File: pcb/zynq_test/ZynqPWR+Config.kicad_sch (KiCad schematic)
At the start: 43 parts, among them SW601 PS_RST, SW602 PROG, U202 XC7Z020-2CLG400I

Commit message: finished diff of HDMI
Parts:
- C601, C604, C605: footprint (none) -> Capacitor_SMD:C_1210_3225Metric
- C632: footprint Capacitor_SMD:C_0402_1005Metric -> Capacitor_SMD:C_1210_3225Metric
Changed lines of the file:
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@@
 			)
 		)
-		(property "Footprint" ""
+		(property "Footprint" "Capacitor_SMD:C_1210_3225Metric"
 			(at 35.2552 83.82 0)
 			(effects
@@
 			)
 		)
-		(property "Footprint" "Capacitor_SMD:C_0402_1005Metric"
+		(property "Footprint" "Capacitor_SMD:C_1210_3225Metric"
 			(at 166.6748 39.37 0)
 			(effects
@@
 			)
 		)
-		(property "Footprint" ""
+		(property "Footprint" "Capacitor_SMD:C_1210_3225Metric"
 			(at 35.2552 62.23 0)
 			(effects
@@
 			)
 		)
-		(property "Footprint" ""
+		(property "Footprint" "Capacitor_SMD:C_1210_3225Metric"
 			(at 17.4752 105.41 0)
 			(effects

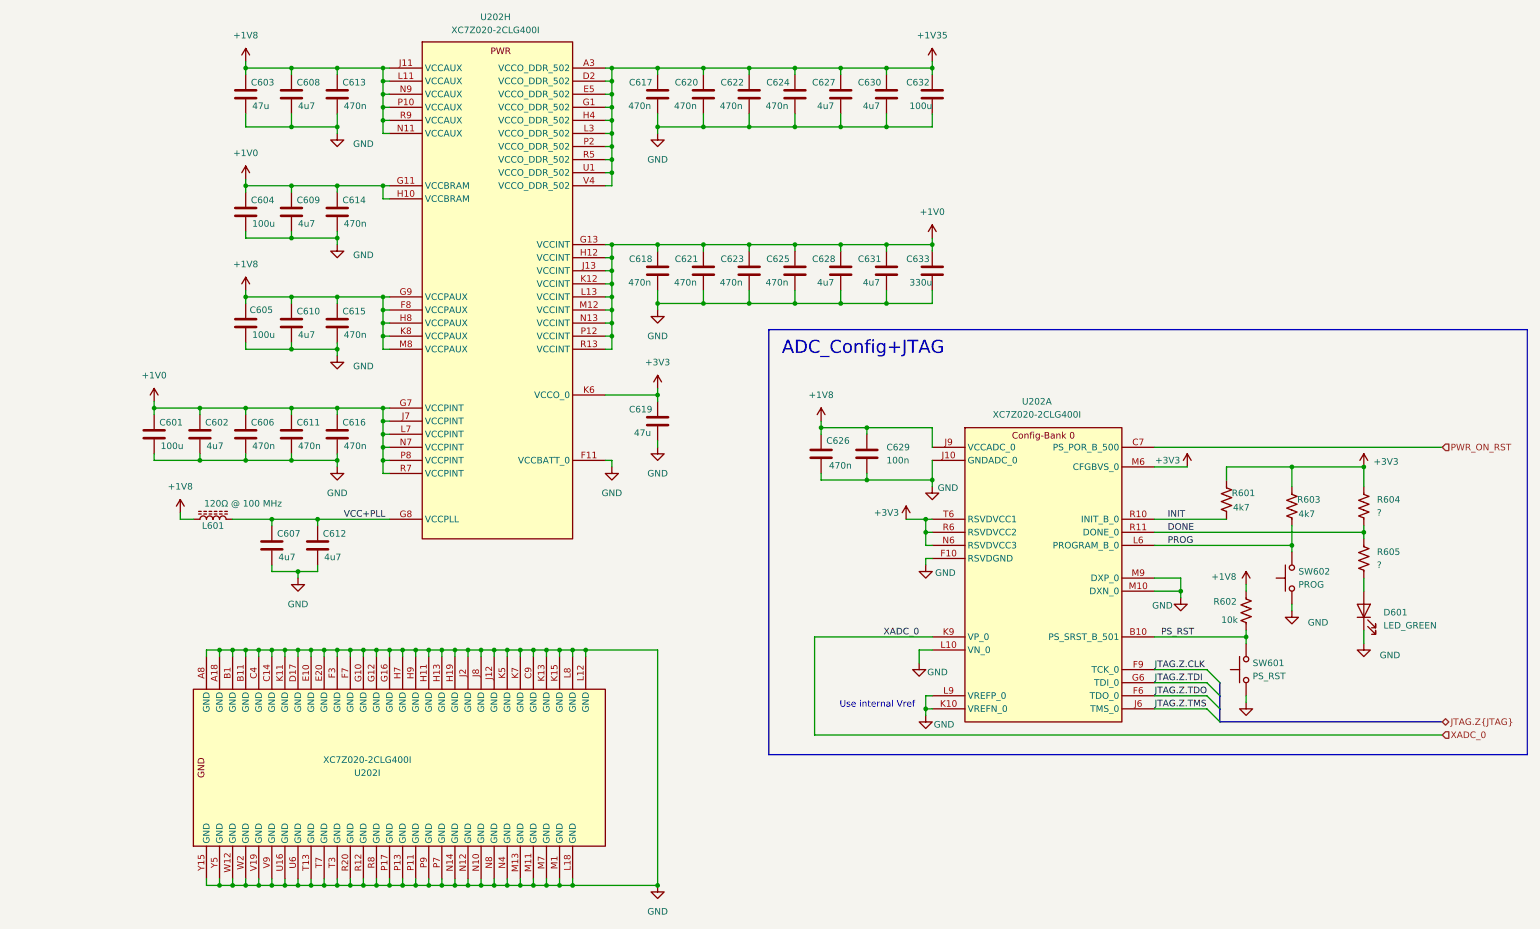
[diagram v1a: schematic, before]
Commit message: Almost done with BOM
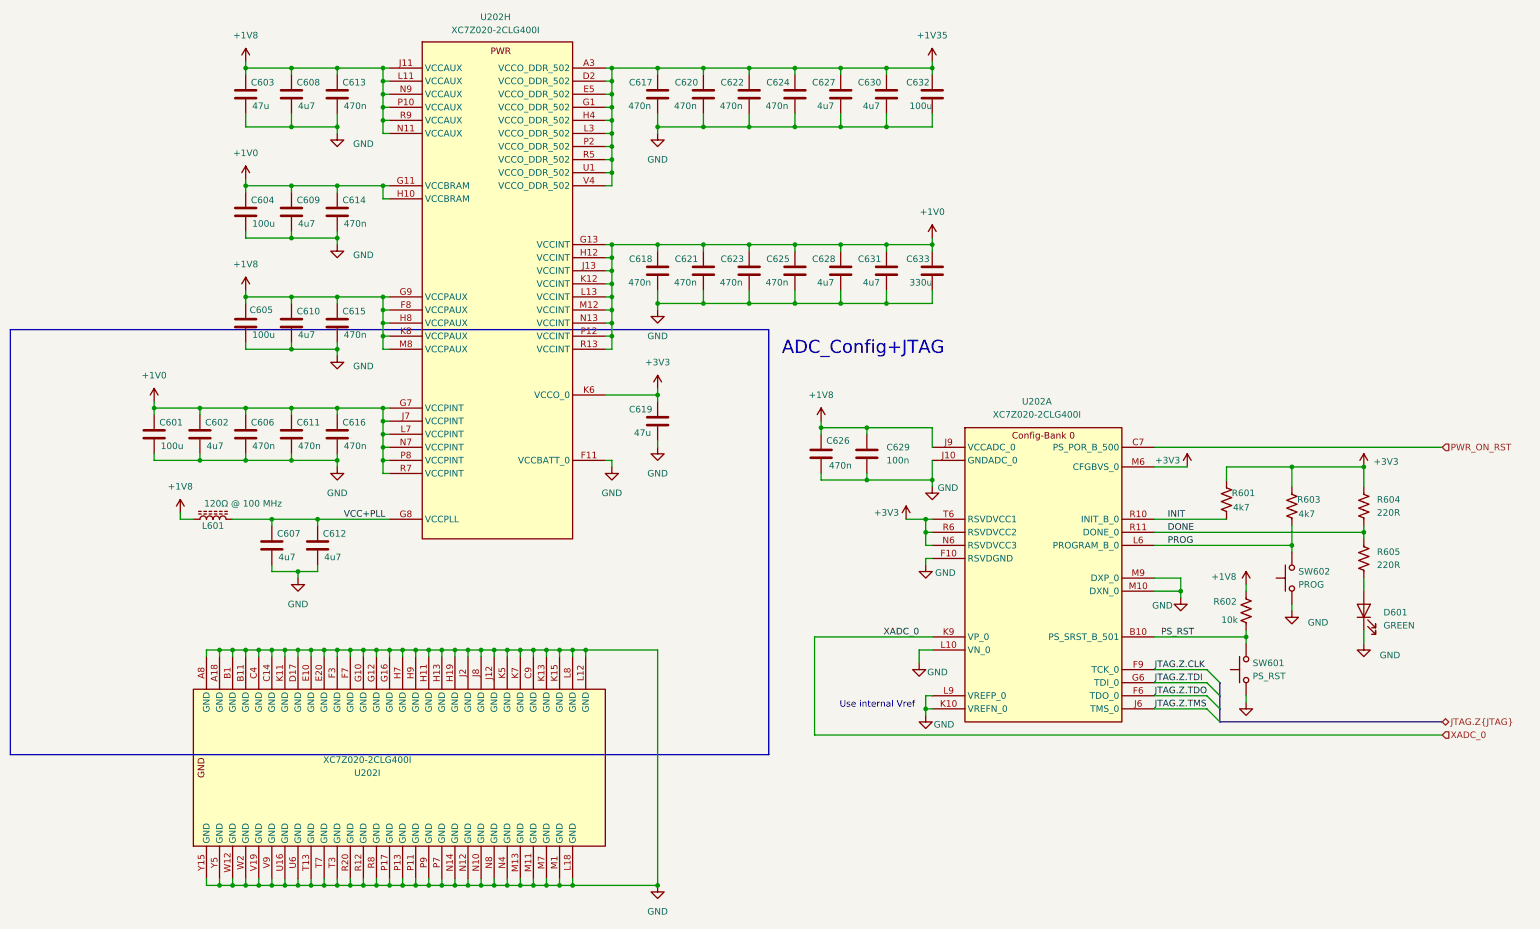
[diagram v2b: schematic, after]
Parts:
- C602, C606, C607, C608, C609, C610, C611, C612, C613, C614, C615, C616, C618, C621, C623, C625, C626, C628, C629, C631: footprint (none) -> Capacitor_SMD:C_0402_1005Metric
- C603, C619, C633: footprint (none) -> Capacitor_SMD:C_1210_3225Metric
- D601: value LED_GREEN -> GREEN; footprint (none) -> LED_SMD:LED_0805_2012Metric
- L601: footprint (none) -> Capacitor_SMD:C_0603_1608Metric
- R601, R602, R603: footprint (none) -> Resistor_SMD:R_0402_1005Metric
- R604, R605: value ? -> 220R; footprint (none) -> Resistor_SMD:R_0402_1005Metric
- SW601, SW602: footprint (none) -> Button_Switch_THT:SW_PUSH_1P1T_6x3.5mm_H4.3_APEM_MJTP1243
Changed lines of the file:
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@@
 	(rectangle
 		(start 135.89 81.28)
-		(end 283.21 163.83)
+		(end -11.43 163.83)
 		(stroke
 			(width 0)
@@
 			)
 		)
-		(property "Value" "?"
+		(property "Value" "220R"
 			(at 254 126.9999 0)
 			(effects
@@
 			)
 		)
-		(property "Footprint" ""
+		(property "Footprint" "Resistor_SMD:R_0402_1005Metric"
 			(at 252.476 125.984 90)
 			(effects
@@
 			)
 		)
-		(property "Footprint" ""
+		(property "Footprint" "Capacitor_SMD:C_0402_1005Metric"
 			(at 155.9052 109.22 0)
 			(effects
@@
 			)
 		)
-		(property "Footprint" ""
+		(property "Footprint" "Button_Switch_THT:SW_PUSH_1P1T_6x3.5mm_H4.3_APEM_MJTP1243"
 			(at 223.52 147.32 0)
 			(effects
@@
 			)
 		)
-		(property "Footprint" ""
+		(property "Footprint" "Capacitor_SMD:C_0402_1005Metric"
 			(at 147.0152 109.22 0)
 			(effects
@@
 			)
 		)
-		(property "Footprint" ""
+		(property "Footprint" "Capacitor_SMD:C_0402_1005Metric"
 			(at 53.0352 105.41 0)
 			(effects
@@
 			)
 		)
-		(property "Footprint" ""
+		(property "Footprint" "Button_Switch_THT:SW_PUSH_1P1T_6x3.5mm_H4.3_APEM_MJTP1243"
 			(at 232.41 129.54 0)
 			(effects
@@
 			)
 		)
-		(property "Footprint" ""
+		(property "Footprint" "Capacitor_SMD:C_0402_1005Metric"
 			(at 140.0048 73.66 0)
 			(effects
@@
 			)
 		)
-		(property "Footprint" ""
+		(property "Footprint" "Capacitor_SMD:C_1210_3225Metric"
 			(at 35.2552 39.37 0)
 			(effects
@@
 			)
 		)
-		(property "Footprint" ""
+		(property "Footprint" "Resistor_SMD:R_0402_1005Metric"
 			(at 225.806 114.554 90)
 			(effects
@@
 			)
 		)
-		(property "Footprint" ""
+		(property "Footprint" "Capacitor_SMD:C_0402_1005Metric"
 			(at 53.0352 39.37 0)
 			(effects
@@
 			)
 		)
-		(property "Footprint" ""
+		(property "Footprint" "Capacitor_SMD:C_0603_1608Metric"
 			(at 27.94 118.11 0)
 			(effects
@@
 			)
 		)
-		(property "Footprint" ""
+		(property "Footprint" "Capacitor_SMD:C_1210_3225Metric"
 			(at 166.6748 73.66 0)
 			(effects
@@
 			)
 		)
-		(property "Footprint" ""
+		(property "Footprint" "Resistor_SMD:R_0402_1005Metric"
 			(at 229.616 136.144 90)
 			(effects
@@
 			)
 		)
-		(property "Footprint" ""
+		(property "Footprint" "Capacitor_SMD:C_0402_1005Metric"
 			(at 49.2252 127 0)
 			(effects
@@
 			)
 		)
-		(property "Footprint" ""
+		(property "Footprint" "Capacitor_SMD:C_0402_1005Metric"
 			(at 44.1452 105.41 0)
 			(effects
@@
 			)
 		)
-		(property "Footprint" ""
+		(property "Footprint" "Capacitor_SMD:C_0402_1005Metric"
 			(at 44.1452 39.37 0)
 			(effects
@@
 			)
 		)
-		(property "Footprint" ""
+		(property "Footprint" "Capacitor_SMD:C_0402_1005Metric"
 			(at 44.1452 83.82 0)
 			(effects
@@
 			)
 		)
-		(property "Footprint" ""
+		(property "Footprint" "Capacitor_SMD:C_0402_1005Metric"
 			(at 148.8948 73.66 0)
 			(effects
@@
 			)
 		)
-		(property "Footprint" ""
+		(property "Footprint" "Capacitor_SMD:C_1210_3225Metric"
 			(at 113.3348 102.87 0)
 			(effects
@@
 			)
 		)
-		(property "Footprint" ""
+		(property "Footprint" "Capacitor_SMD:C_0402_1005Metric"
 			(at 35.2552 105.41 0)
 			(effects
@@
 			)
 		)
-		(property "Footprint" ""
+		(property "Footprint" "Capacitor_SMD:C_0402_1005Metric"
 			(at 131.1148 73.66 0)
 			(effects
@@
 			)
 		)
-		(property "Footprint" ""
+		(property "Footprint" "Resistor_SMD:R_0402_1005Metric"
 			(at 238.506 115.824 90)
 			(effects
@@
 			)
 		)
-		(property "Footprint" ""
+		(property "Footprint" "Capacitor_SMD:C_0402_1005Metric"
 			(at 157.7848 73.66 0)
 			(effects
@@
 			)
 		)
-		(property "Footprint" ""
+		(property "Footprint" "Capacitor_SMD:C_0402_1005Metric"
 			(at 113.3348 73.66 0)
 			(effects
@@
 			)
 		)
-		(property "Footprint" ""
+		(property "Footprint" "Capacitor_SMD:C_0402_1005Metric"
 			(at 40.3352 127 0)
 			(effects
@@
 			)
 		)
-		(property "Value" "LED_GREEN"
+		(property "Value" "GREEN"
 			(at 255.27 138.7474 90)
 			(effects
@@
 			)
 		)
-		(property "Footprint" ""
+		(property "Footprint" "LED_SMD:LED_0805_2012Metric"
 			(at 251.46 135.89 0)
 			(effects
@@
 			)
 		)
-		(property "Footprint" ""
+		(property "Footprint" "Capacitor_SMD:C_0402_1005Metric"
 			(at 53.0352 62.23 0)
 			(effects
@@
 			)
 		)
-		(property "Footprint" ""
+		(property "Footprint" "Capacitor_SMD:C_0402_1005Metric"
 			(at 44.1452 62.23 0)
 			(effects
@@
 			)
 		)
-		(property "Footprint" ""
+		(property "Footprint" "Capacitor_SMD:C_0402_1005Metric"
 			(at 26.3652 105.41 0)
 			(effects
@@
 			)
 		)
-		(property "Value" "?"
+		(property "Value" "220R"
 			(at 254 116.8399 0)
 			(effects
@@
 			)
 		)
-		(property "Footprint" ""
+		(property "Footprint" "Resistor_SMD:R_0402_1005Metric"
 			(at 252.476 115.824 90)
 			(effects
@@
 			)
 		)
-		(property "Footprint" ""
+		(property "Footprint" "Capacitor_SMD:C_0402_1005Metric"
 			(at 53.0352 83.82 0)
 			(effects
@@
 			)
 		)
-		(property "Footprint" ""
+		(property "Footprint" "Capacitor_SMD:C_0402_1005Metric"
 			(at 122.2248 73.66 0)
 			(effects
